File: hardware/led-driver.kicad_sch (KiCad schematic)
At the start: 22 parts, among them J101 BM04B-SRSS-TB, J102 BM04B-SRSS-TB, J103 VH_S2P-VH, U101 PCA9685PW_118

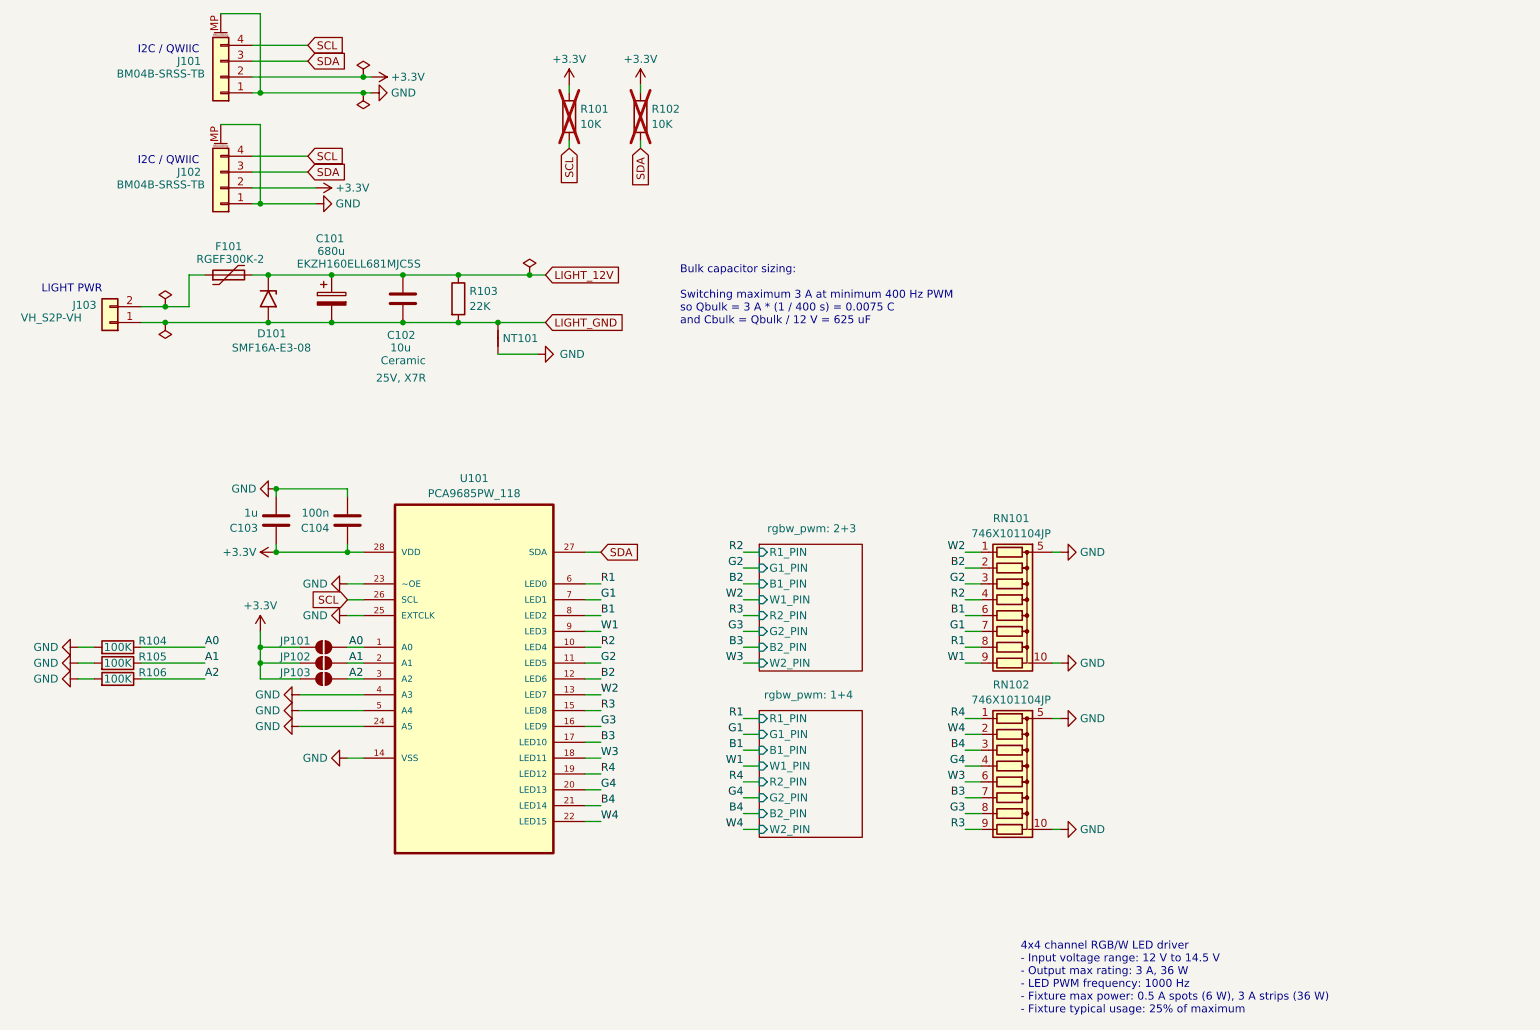
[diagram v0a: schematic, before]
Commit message: Tidy up the schematic.
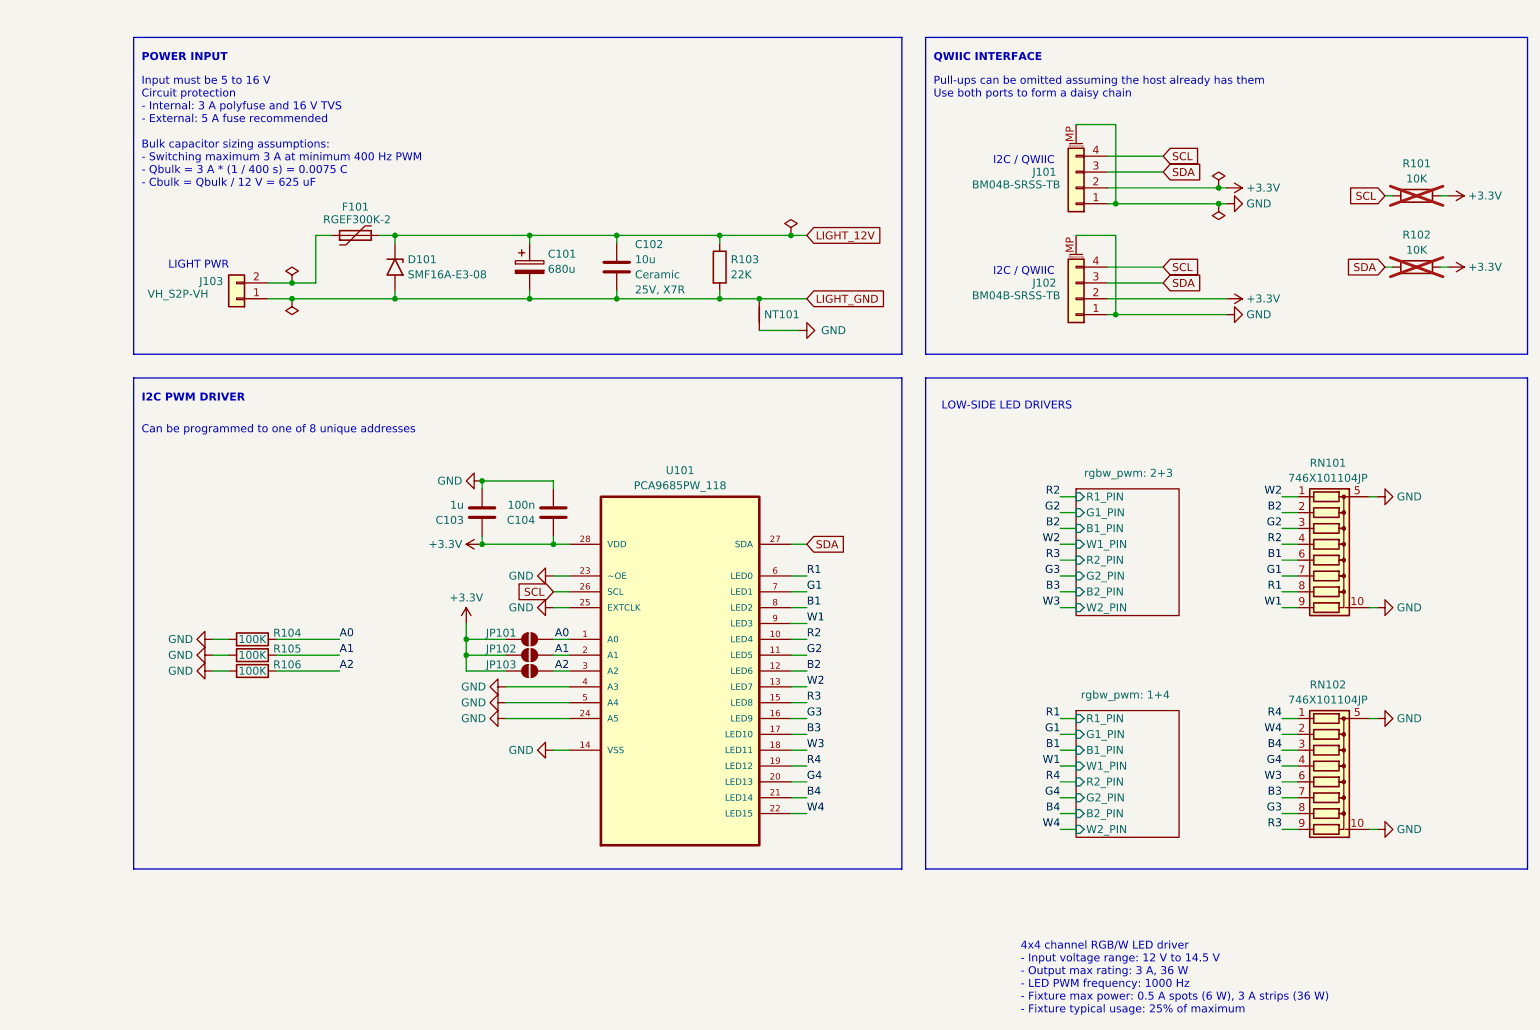
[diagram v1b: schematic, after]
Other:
- note added: "Can be programmed to one of 8 unique addresses"
- note added: "I2C PWM DRIVER"
- note added: "Input must be 5 to 16 V Circuit protection - Internal: 3 A polyfuse and 16 V TVS - External: 5 A fuse recommended Bulk capacitor sizing assumptions: - Switching maximum 3 A at minimum 400 Hz PWM - Qbulk = 3 A * (1 / 400 s) = 0.0075 C - Cbulk = Qbulk / 12 V = 625 uF"
- note added: "LOW-SIDE LED DRIVERS"
- note added: "POWER INPUT"
- note added: "Pull-ups can be omitted assuming the host already has them Use both ports to form a daisy chain"
- note added: "QWIIC INTERFACE"
- note removed: "Bulk capacitor sizing: Switching maximum 3 A at minimum 400 Hz PWM so Qbulk = 3 A * (1 / 400 s) = 0.0075 C and Cbulk = Qbulk / 12 V = 625 uF"
- moved on the sheet: C101, C102, C103, C104, D101, F101, J101, J102, J103, JP101, JP102, JP103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
